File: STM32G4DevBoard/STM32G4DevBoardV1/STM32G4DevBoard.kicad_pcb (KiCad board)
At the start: 4 copper layers, 44.7 x 23.5 mm, 29 parts, among them J1 USB_B_Micro, J2 Conn_01x13, J3 Conn_01x13, U1 STM32G431KBTx, U2 LD3985M33R_SOT23, Y1 24MHz

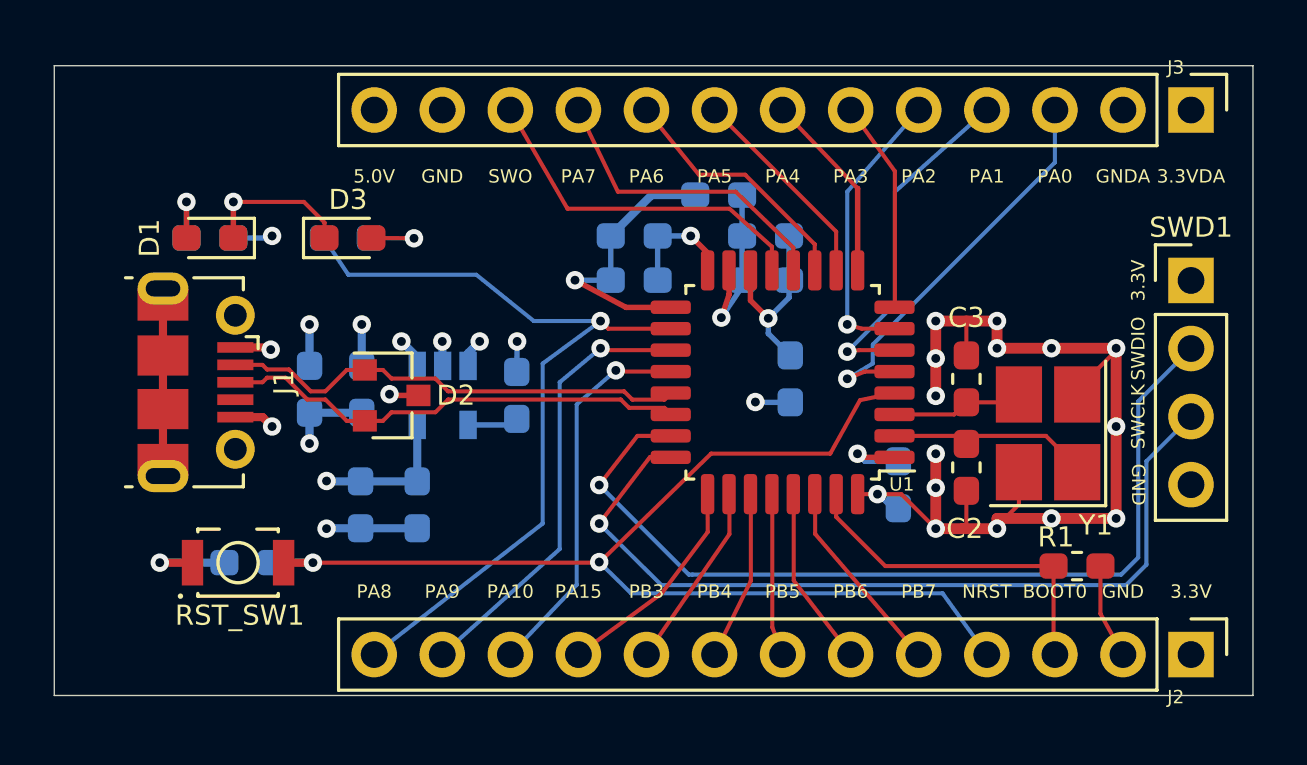
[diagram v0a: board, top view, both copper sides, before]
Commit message: Last minute tweak, adjustment
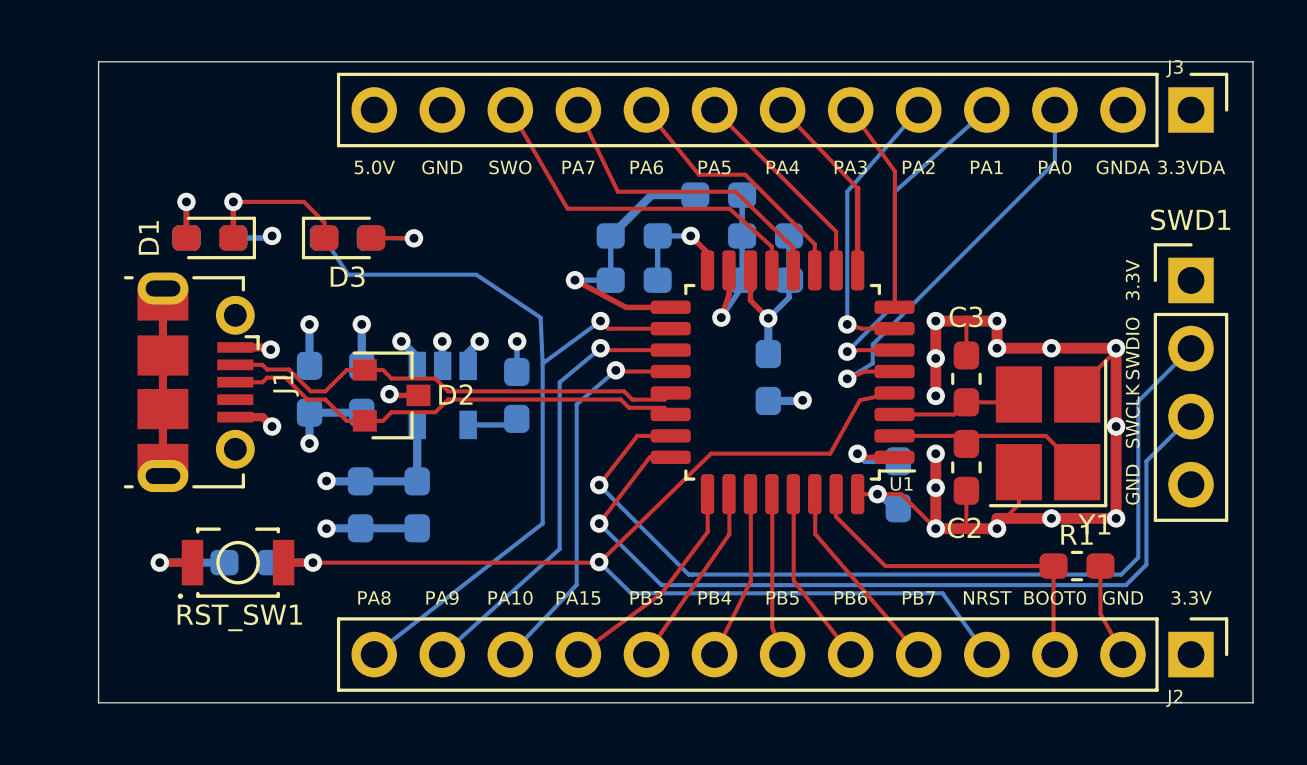
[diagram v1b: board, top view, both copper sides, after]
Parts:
- moved FB2 0.82 mm to (131.8, 91.1)
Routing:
- net PA8: track 31.0 -> 30.4 mm
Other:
- board size 44.7 x 23.5 mm -> 43.1 x 23.9 mm
